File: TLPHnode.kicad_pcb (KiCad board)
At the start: 4 copper layers, 28 x 20.5 mm, 29 parts, among them P1 Bat, P2 CONN_01X05, SW1 Reset, U1 NCP703, U2 LD39130S, U3 LPS25HB, U4 Si7006-A20, U5 ESP-12E, U6 ISL29035

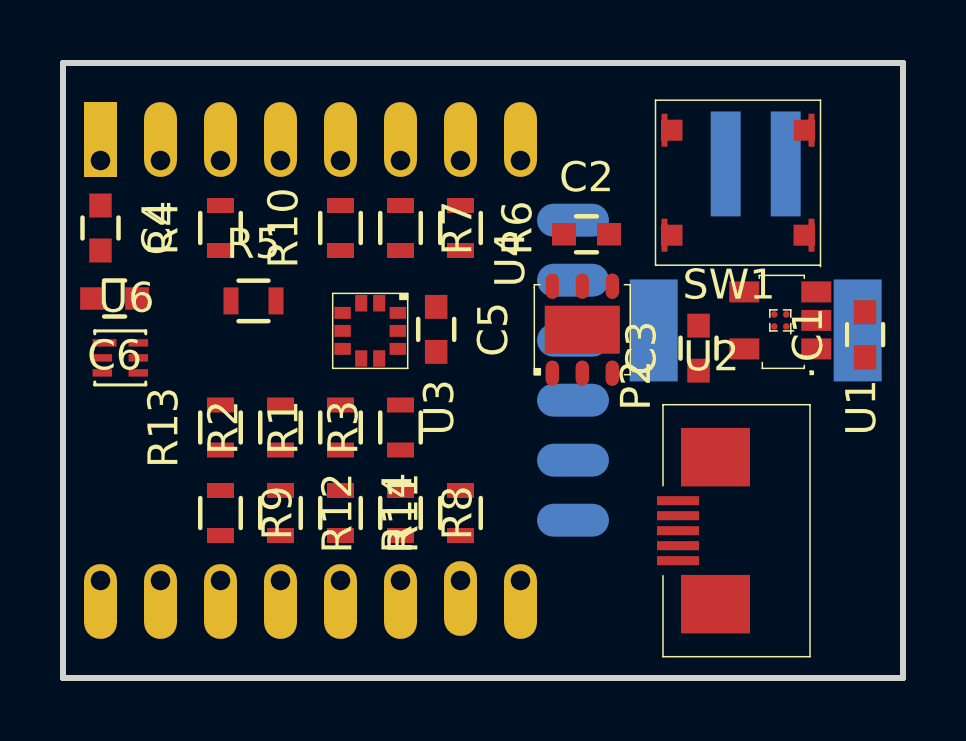
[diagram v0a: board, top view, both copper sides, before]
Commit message: Check-point: layout passes DRM, References visible
On branch master
modified:   TLPHnode-cache.lib
modified:   TLPHnode.kicad_pcb
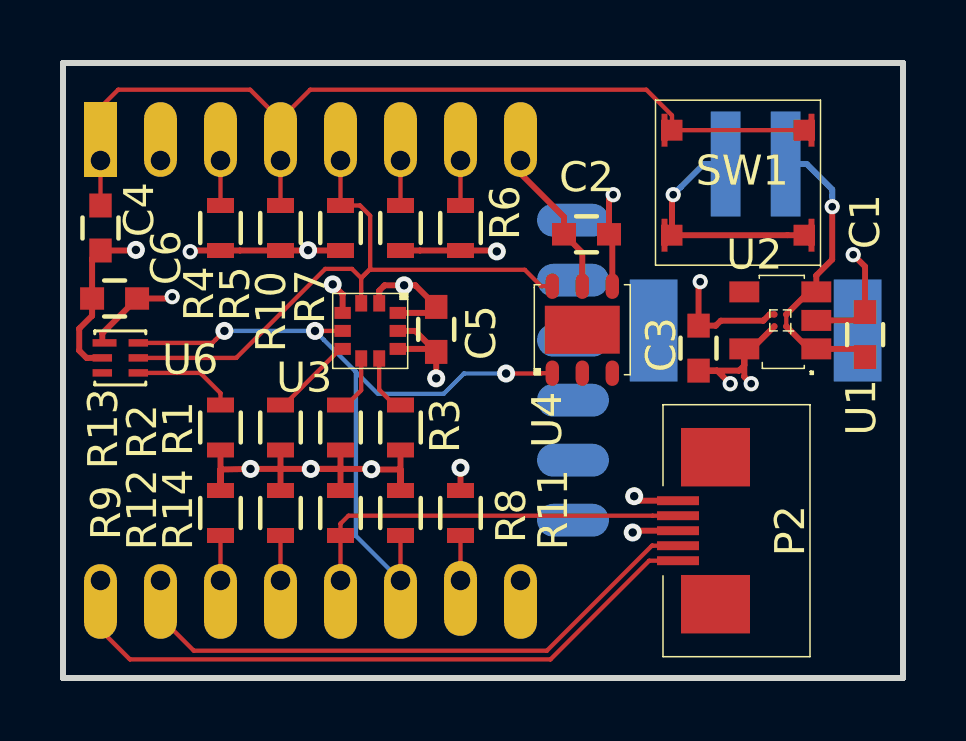
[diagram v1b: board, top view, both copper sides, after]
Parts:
- moved R5 2.59 mm to (137.8, 86.0), turned to 90 degrees
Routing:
- net VCC: track 0.00 -> 42.1 mm, vias 0 -> 11
- net Net-(C4-Pad1): track 0.00 -> 32.4 mm
- net GND: track 0.00 -> 31.7 mm, vias 0 -> 9
- net /I2C_SDA: track 0.00 -> 25.1 mm, vias 0 -> 3
- net /TXD: track 0.00 -> 22.7 mm
- net /I2C_SCL: track 0.00 -> 21.2 mm
- net /RXD: track 0.00 -> 20.4 mm
- net /PGM: track 0.00 -> 13.3 mm
- net Net-(C1-Pad1): track 0.00 -> 10.3 mm, vias 0 -> 1
- net Net-(R13-Pad2): track 0.00 -> 3.41 mm
- net Net-(R2-Pad2): track 0.00 -> 2.84 mm
- net Net-(R3-Pad2): track 0.00 -> 1.96 mm
- net Net-(R1-Pad2): track 0.00 -> 1.95 mm
- net Net-(R9-Pad2): track 0.00 -> 1.50 mm
- net Net-(R7-Pad1): track 0.00 -> 1.50 mm
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- added copper zone on In1.Cu.GND, net GND
- added copper zone on In2.Cu.VCC, net VCC
